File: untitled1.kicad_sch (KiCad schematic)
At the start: 25 parts, among them J14 Conn_01x20_MountingPin, J16 HC-05 Breakout Board, J3 Conn_01x02_Pin, J4 Conn_01x02_Pin, J7 Conn_01x20_MountingPin, J9 Conn_01x20_MountingPin, SW2 SW_Push, SW3 SW_Push, SW4 SW_Push, SW8 SW_SPDT

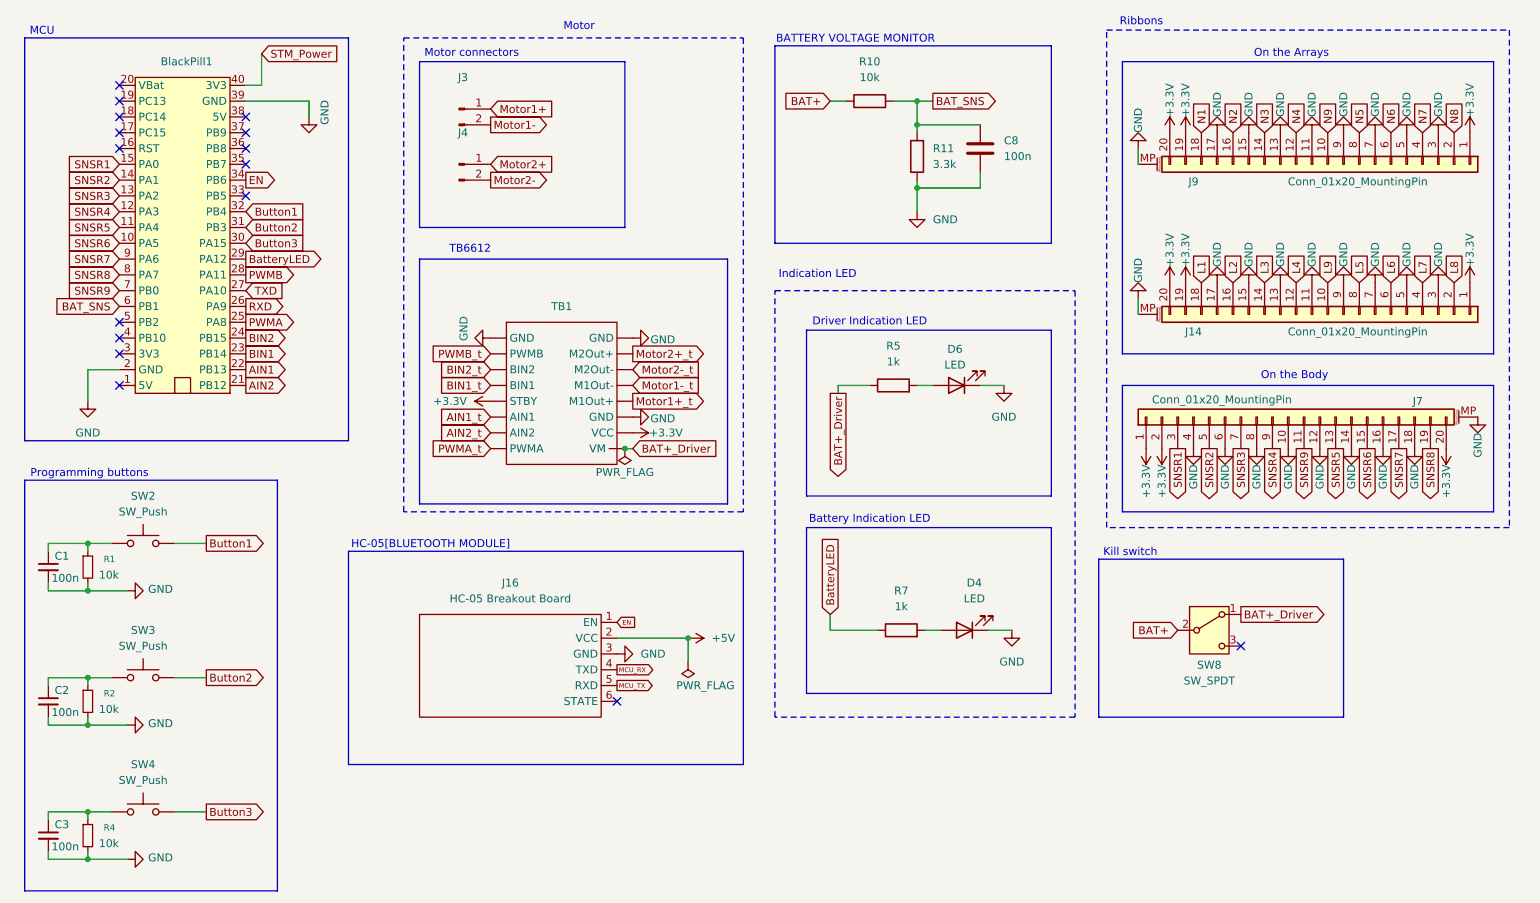
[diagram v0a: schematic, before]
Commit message: PCB
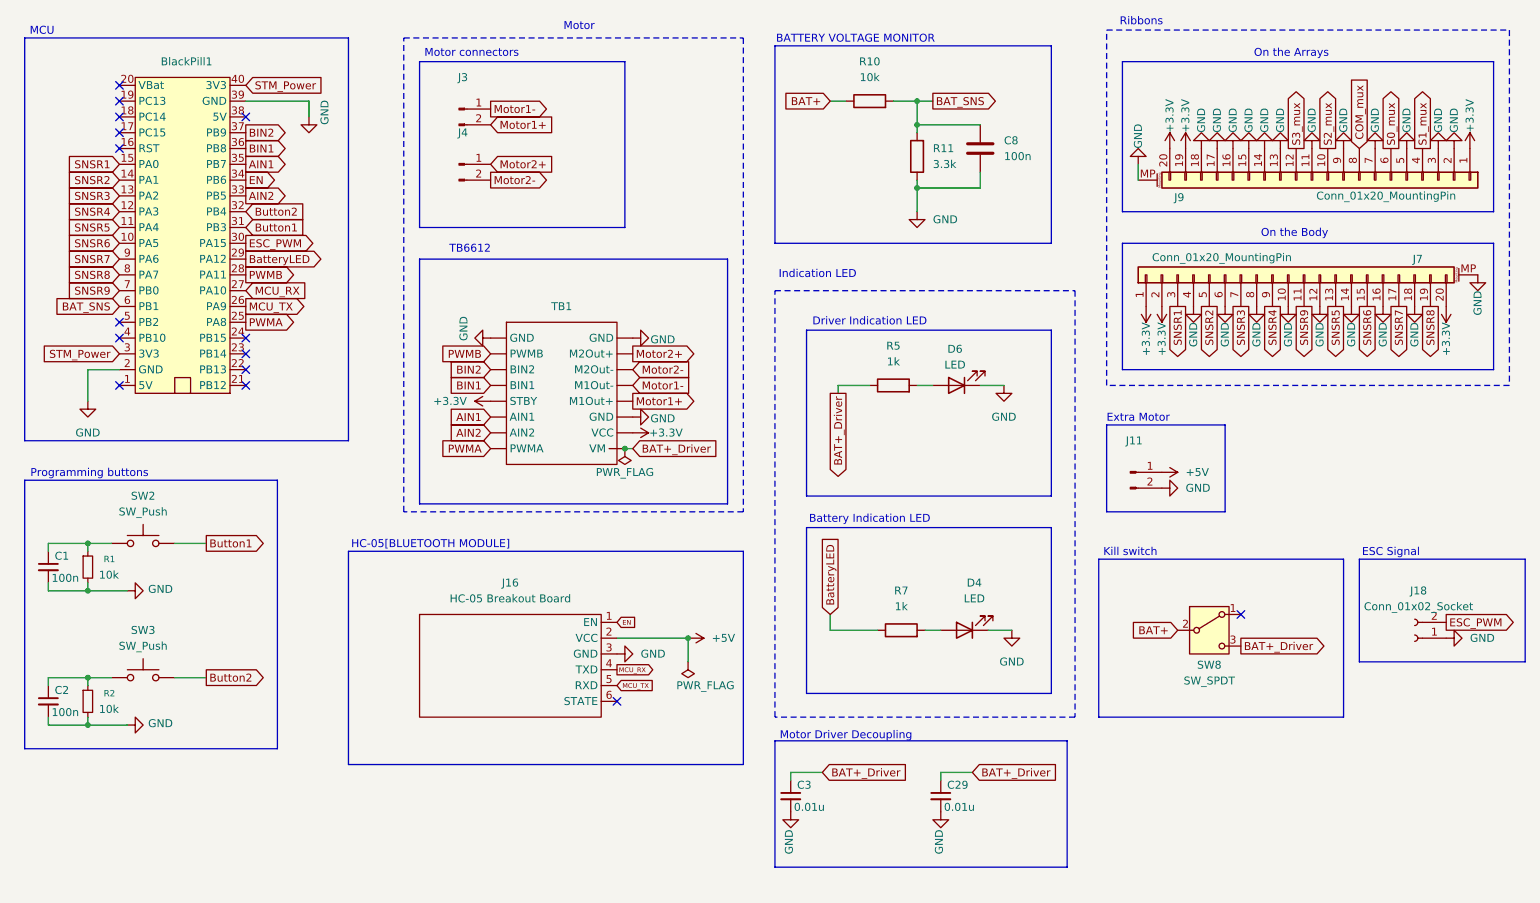
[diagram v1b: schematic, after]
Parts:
- removed J14: Conn_01x20_MountingPin, Connector_FFC-FPC:Amphenol_F32Q-1A7x1-11020_1x20-1MP_P0.5mm_Horizontal, symbol Connector_Generic_MountingPin:Conn_01x20_MountingPin
- removed R4: 10k, Resistor_SMD:R_0603_1608Metric_Pad0.98x0.95mm_HandSolder, symbol Device:R_Small
- removed SW4: SW_Push, customs:Push button-fp, symbol Switch:SW_Push
- added C29: 0.01u, Capacitor_SMD:C_0603_1608Metric_Pad1.08x0.95mm_HandSolder, symbol Device:C_Small
- added J11: Conn_01x02_Pin, Connector_PinHeader_2.00mm:PinHeader_1x02_P2.00mm_Vertical, symbol Connector:Conn_01x02_Pin
- added J18: Conn_01x02_Socket, Connector_JST:JST_PH_B2B-PH-K_1x02_P2.00mm_Vertical, symbol Connector:Conn_01x02_Socket
- BlackPill1: footprint customs:blackpill_fp -> CustomLibrary:blackpill_fp
- C3: value 100n -> 0.01u
- D4, D6: footprint LED_THT:LED_D3.0mm -> LED_SMD:LED_0603_1608Metric_Pad1.05x0.95mm_HandSolder
- SW2, SW3: footprint customs:Push button-fp -> CustomLibrary:Push button-fp
- TB1: footprint customs:TB6612 module -> CustomLibrary:TB6612 module
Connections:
- net AIN1_t is gone; now on net AIN1: TB1.6 (AIN1)
- net AIN2_t is gone; now on net AIN2: TB1.7 (AIN2)
- net BIN1_t is gone; now on net BIN1: TB1.4 (BIN1)
- net BIN2_t is gone; now on net BIN2: TB1.3 (BIN2)
- net Motor1+_t is gone; now on net Motor1+: TB1.13 (M1Out+)
- net Motor1-_t is gone; now on net Motor1-: TB1.12 (M1Out-)
- net Motor2+_t is gone; now on net Motor2+: TB1.10 (M2Out+)
- net Motor2-_t is gone; now on net Motor2-: TB1.11 (M2Out-)
- net N1 is gone; now on net GND: J9.18 (Pin_18)
- net N2 is gone; now on net GND: J9.16 (Pin_16)
- net N3 is gone; now on net GND: J9.14 (Pin_14)
- net N8 is gone; now on net GND: J9.2 (Pin_2)
- net PWMA_t is gone; now on net PWMA: TB1.8 (PWMA)
- net PWMB_t is gone; now on net PWMB: TB1.2 (PWMB)
- net RXD is gone; now on net MCU_TX: BlackPill1.26 (PA9)
- net TXD is gone; now on net MCU_RX: BlackPill1.27 (PA10)
- net +5V: now also J11.1 (Pin_1)
- net AIN1: now also BlackPill1.35 (PB7); no longer BlackPill1.22 (PB13)
- net AIN2: now also BlackPill1.33 (PB5); no longer BlackPill1.21 (PB12)
- net BAT+_Driver: now also C3.1, SW8.3 (C), C29.1; no longer SW8.1 (A)
- net BIN1: now also BlackPill1.36 (PB8); no longer BlackPill1.23 (PB14)
- net BIN2: now also BlackPill1.37 (PB9); no longer BlackPill1.24 (PB15)
- net Button1: now also BlackPill1.31 (PB3); no longer BlackPill1.32 (PB4)
- net Button2: now also BlackPill1.32 (PB4); no longer BlackPill1.31 (PB3)
- net GND: now also C29.2, J11.2 (Pin_2), J18.1 (Pin_1)
- net Motor1+: now also J3.2 (Pin_2); no longer J3.1 (Pin_1)
- net Motor1-: now also J3.1 (Pin_1); no longer J3.2 (Pin_2)
- net STM_Power: now also BlackPill1.3 (3V3)
- net Button3 renamed ESC_PWM
- net ESC_PWM: now also J18.2 (Pin_2)
- net N4 renamed S3_mux
- net N5 renamed COM_mux
- net N6 renamed S0_mux
- net N7 renamed S1_mux
- net N9 renamed S2_mux
- no-connect marks 16 -> 15
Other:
- note added: "ESC Signal"
- note added: "Extra Motor"
- note added: "Motor Driver Decoupling"
- moved on the sheet: J7
